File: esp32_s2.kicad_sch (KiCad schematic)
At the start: 15 parts, among them U3 ESP32-S2-MINI-2U-N4

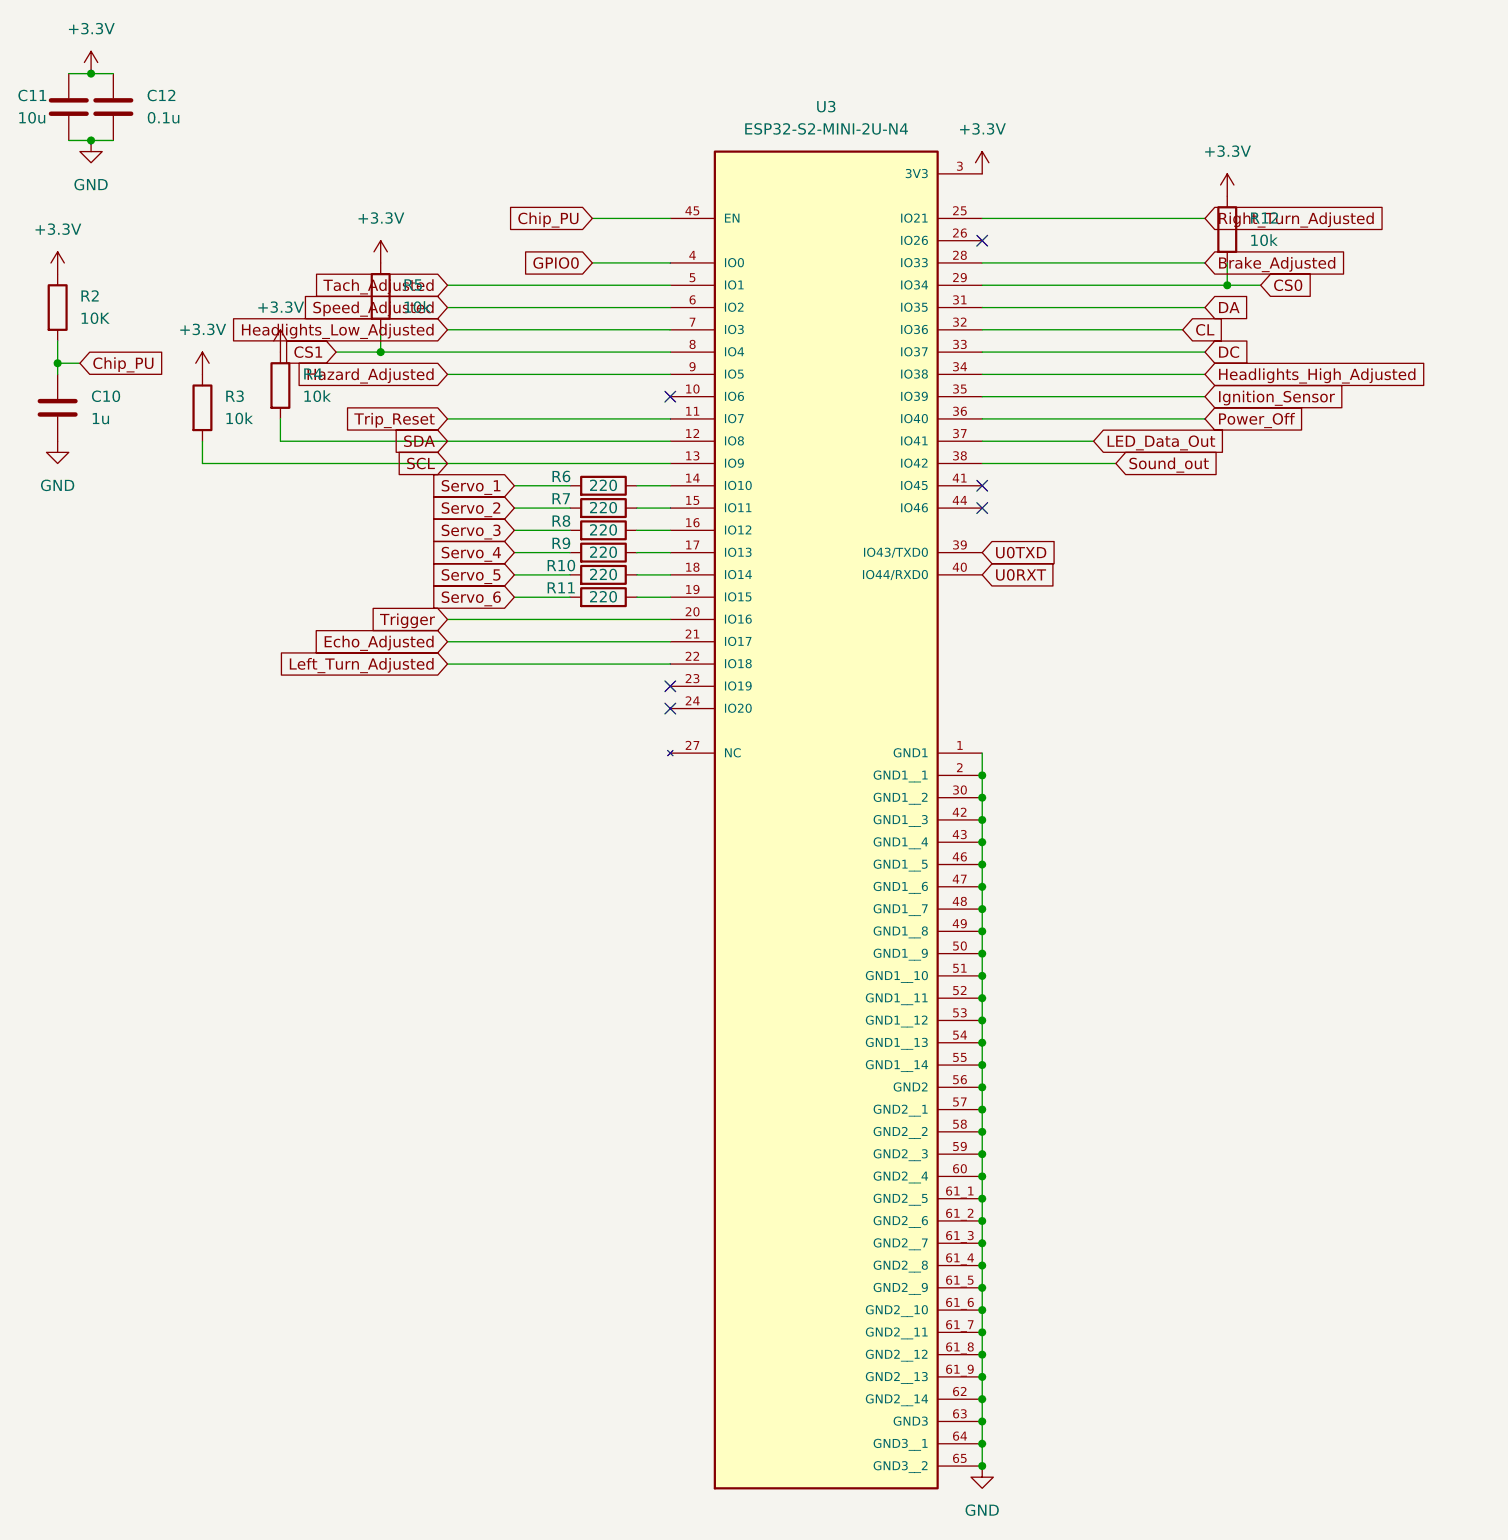
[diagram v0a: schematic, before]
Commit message: Update
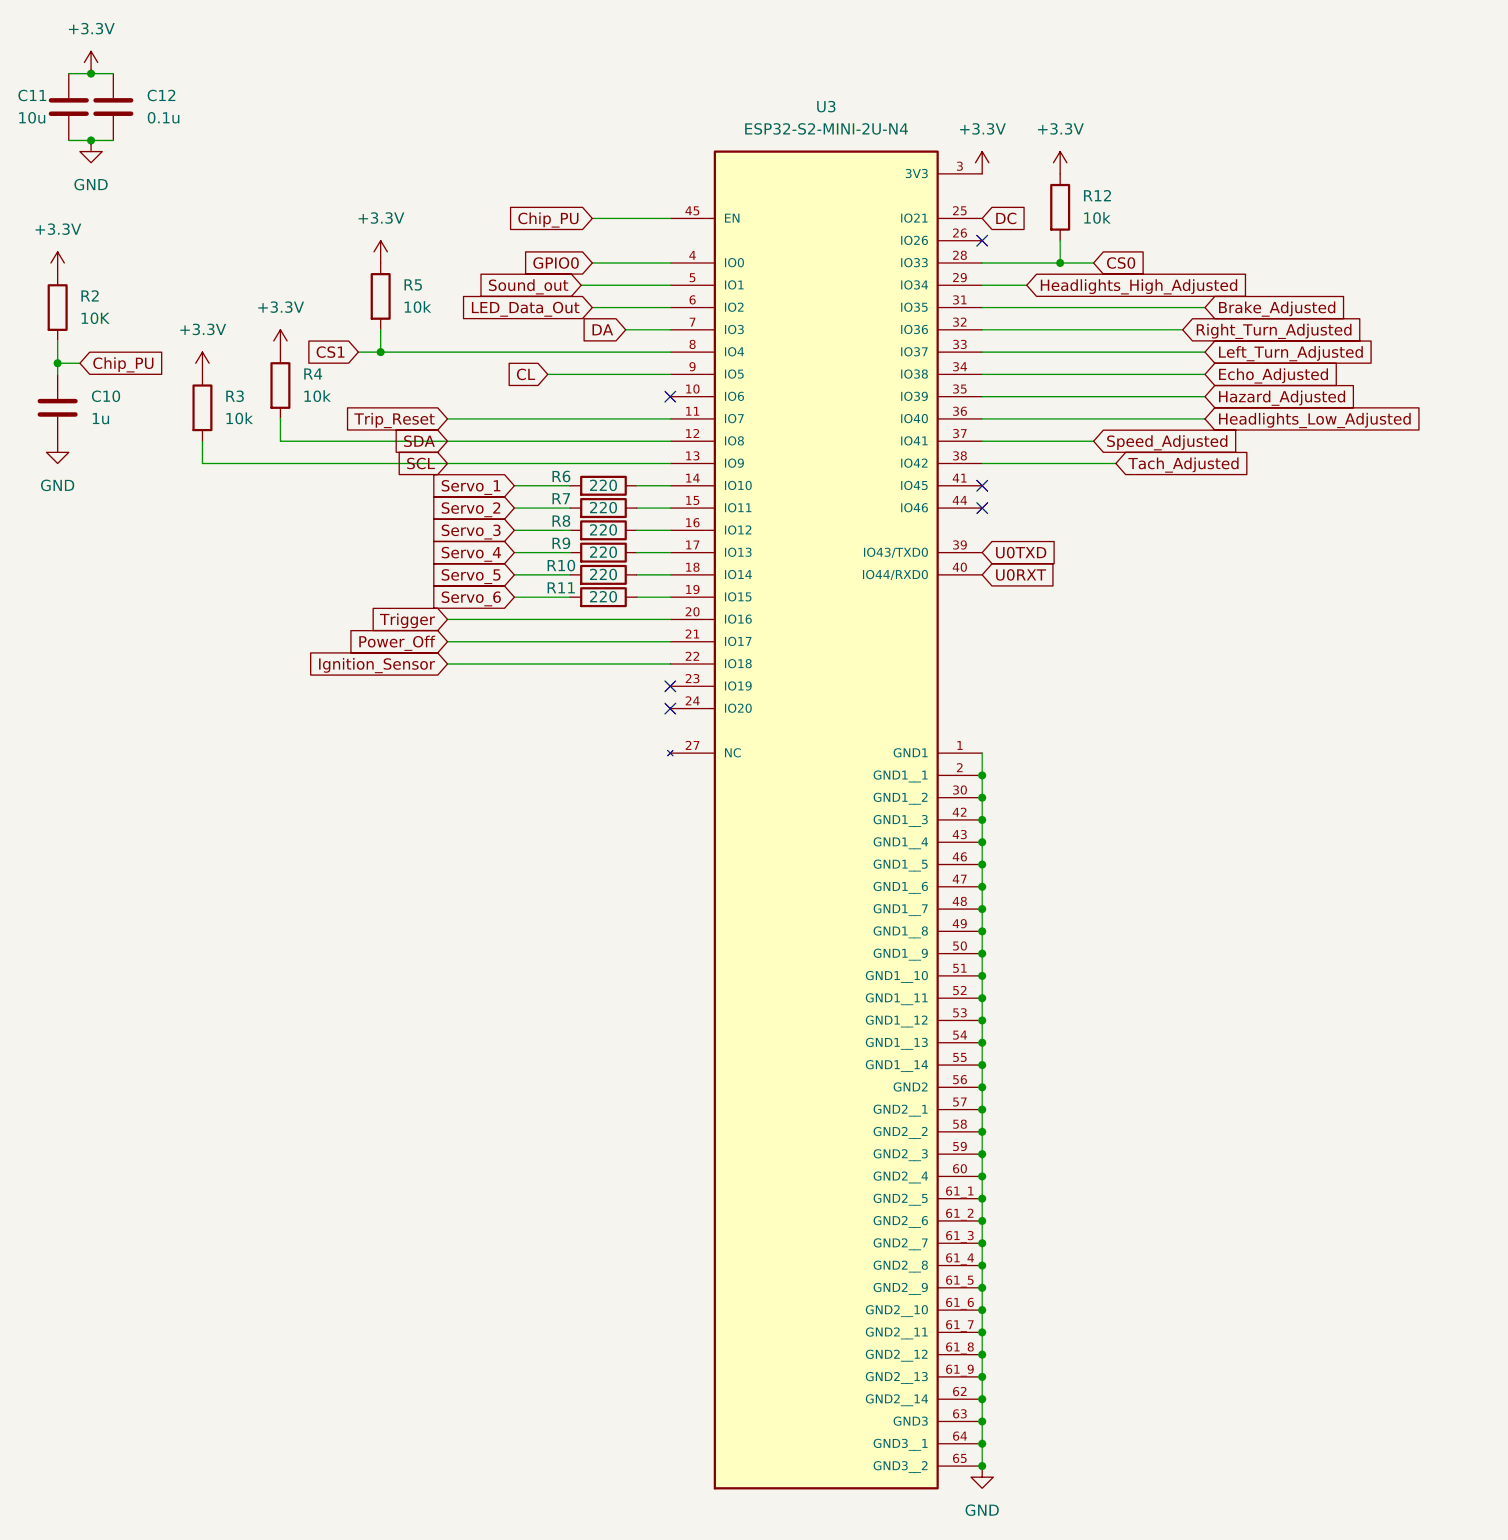
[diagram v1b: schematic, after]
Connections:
- net Brake_Adjusted: now also U3.31 (IO35); no longer U3.28 (IO33)
- net CL: now also U3.9 (IO5); no longer U3.32 (IO36)
- net CS0: now also U3.28 (IO33); no longer U3.29 (IO34)
- net DA: now also U3.7 (IO3); no longer U3.31 (IO35)
- net DC: now also U3.25 (IO21); no longer U3.33 (IO37)
- net Echo_Adjusted: now also U3.34 (IO38); no longer U3.21 (IO17)
- net Hazard_Adjusted: now also U3.35 (IO39); no longer U3.9 (IO5)
- net Headlights_High_Adjusted: now also U3.29 (IO34); no longer U3.34 (IO38)
- net Headlights_Low_Adjusted: now also U3.36 (IO40); no longer U3.7 (IO3)
- net Ignition_Sensor: now also U3.22 (IO18); no longer U3.35 (IO39)
- net LED_Data_Out: now also U3.6 (IO2); no longer U3.37 (IO41)
- net Left_Turn_Adjusted: now also U3.33 (IO37); no longer U3.22 (IO18)
- net Power_Off: now also U3.21 (IO17); no longer U3.36 (IO40)
- net Right_Turn_Adjusted: now also U3.32 (IO36); no longer U3.25 (IO21)
- net Sound_out: now also U3.5 (IO1); no longer U3.38 (IO42)
- net Speed_Adjusted: now also U3.37 (IO41); no longer U3.6 (IO2)
- net Tach_Adjusted: now also U3.38 (IO42); no longer U3.5 (IO1)
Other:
- moved on the sheet: R12

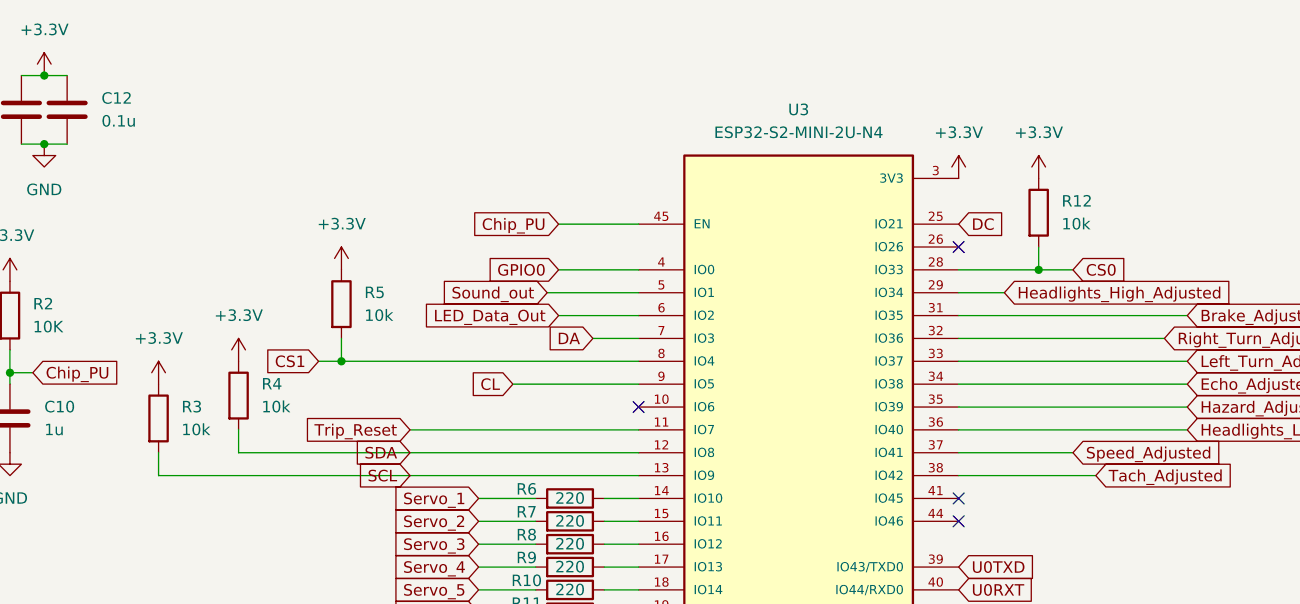
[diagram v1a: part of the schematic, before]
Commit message: update
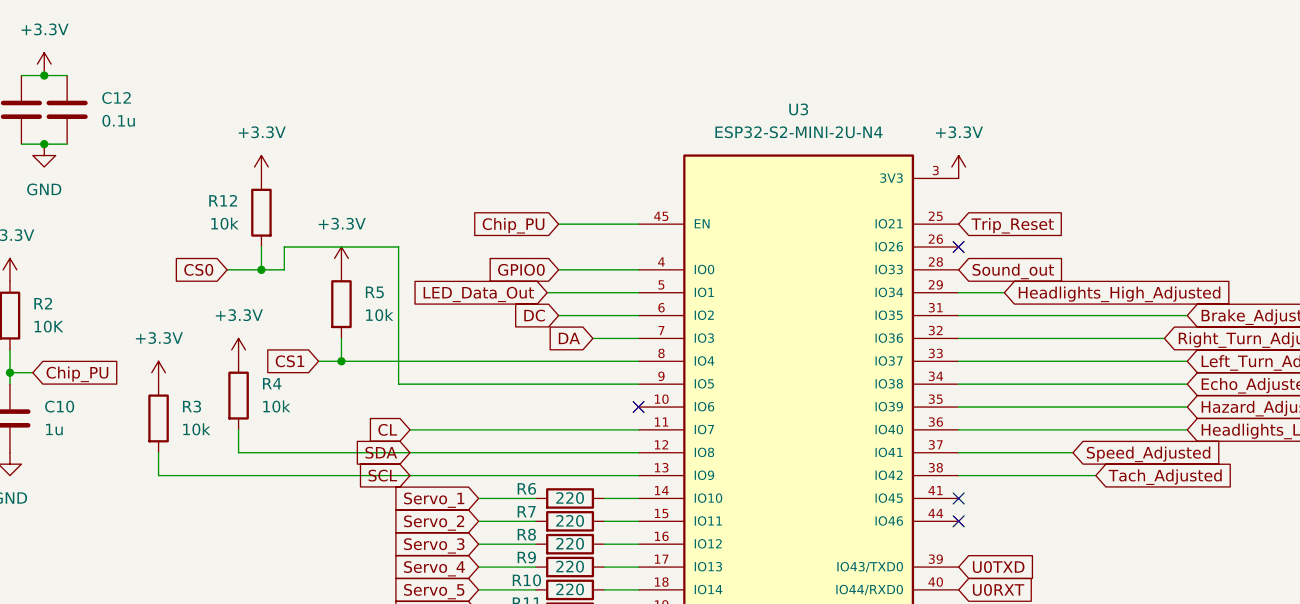
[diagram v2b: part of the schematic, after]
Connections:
- net CL: now also U3.11 (IO7); no longer U3.9 (IO5)
- net CS0: now also U3.9 (IO5); no longer U3.28 (IO33)
- net DC: now also U3.6 (IO2); no longer U3.25 (IO21)
- net LED_Data_Out: now also U3.5 (IO1); no longer U3.6 (IO2)
- net Sound_out: now also U3.28 (IO33); no longer U3.5 (IO1)
- net Trip_Reset: now also U3.25 (IO21); no longer U3.11 (IO7)
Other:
- moved on the sheet: R12
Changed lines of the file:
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@@
 	)
 	(junction
-		(at 132.08 43.18)
-		(diameter 0)
-		(color 0 0 0 0)
-	)
-	(junction
 		(at 123.19 160.02)
 		(diameter 0)
@@
 	)
 	(junction
+		(at 45.72 43.18)
+		(diameter 0)
+		(color 0 0 0 0)
+	)
+	(junction
 		(at 123.19 134.62)
 		(diameter 0)
@@
 	(wire
 		(pts
+			(xy 45.72 43.18) (xy 48.26 43.18)
+		)
+		(stroke
+			(width 0)
+			(type default)
+		)
+	)
+	(wire
+		(pts
 			(xy 123.19 147.32) (xy 123.19 149.86)
 		)
@@
 	(wire
 		(pts
-			(xy 73.66 55.88) (xy 87.63 55.88)
+			(xy 48.26 40.64) (xy 48.26 43.18)
 		)
 		(stroke
@@
 	(wire
 		(pts
-			(xy 132.08 43.18) (xy 123.19 43.18)
+			(xy 60.96 55.88) (xy 60.96 40.64)
 		)
 		(stroke
@@
 	(wire
 		(pts
+			(xy 60.96 40.64) (xy 48.26 40.64)
+		)
+		(stroke
+			(width 0)
+			(type default)
+		)
+	)
+	(wire
+		(pts
 			(xy 128.27 45.72) (xy 123.19 45.72)
 		)
@@
 	(wire
 		(pts
-			(xy 132.08 43.18) (xy 135.89 43.18)
+			(xy 41.91 43.18) (xy 45.72 43.18)
 		)
 		(stroke
@@
 	(wire
 		(pts
-			(xy 132.08 40.64) (xy 132.08 43.18)
+			(xy 60.96 55.88) (xy 87.63 55.88)
 		)
 		(stroke
@@
 		)
 	)
+	(wire
+		(pts
+			(xy 45.72 40.64) (xy 45.72 43.18)
+		)
+		(stroke
+			(width 0)
+			(type default)
+		)
+	)
 	(global_label "Right_Turn_Adjusted"
 		(shape input)
@@
 	(global_label "Trip_Reset"
 		(shape input)
-		(at 62.23 60.96 180)
+		(at 123.19 38.1 0)
 		(fields_autoplaced yes)
 		(effects
@@
 				(size 1.27 1.27)
 			)
-			(justify right)
+			(justify left)
 		)
 		(property "Intersheetrefs" "${INTERSHEET_REFS}"
-			(at 49.5686 60.96 0)
+			(at 135.8514 38.1 0)
 			(hide yes)
 			(show_name no)
@@
 					(size 1.27 1.27)
 				)
-				(justify right)
+				(justify left)
 			)
 		)
@@
 	(global_label "Sound_out"
 		(shape input)
-		(at 77.47 45.72 180)
+		(at 123.19 43.18 0)
 		(fields_autoplaced yes)
 		(effects
@@
 				(size 1.27 1.27)
 			)
-			(justify right)
+			(justify left)
 		)
 		(property "Intersheetrefs" "${INTERSHEET_REFS}"
-			(at 64.688 45.72 0)
+			(at 135.972 43.18 0)
 			(hide yes)
 			(show_name no)
@@
 					(size 1.27 1.27)
 				)
-				(justify right)
+				(justify left)
 			)
 		)
@@
 	(global_label "LED_Data_Out"
 		(shape input)
-		(at 78.74 48.26 180)
+		(at 77.47 45.72 180)
 		(fields_autoplaced yes)
 		(effects
@@
 		)
 		(property "Intersheetrefs" "${INTERSHEET_REFS}"
-			(at 62.8736 48.26 0)
+			(at 61.6036 45.72 0)
 			(hide yes)
 			(show_name no)
@@
 	(global_label "CL"
 		(shape input)
-		(at 73.66 55.88 180)
+		(at 62.23 60.96 180)
 		(fields_autoplaced yes)
 		(effects
@@
 		)
 		(property "Intersheetrefs" "${INTERSHEET_REFS}"
-			(at 68.3767 55.88 0)
+			(at 56.9467 60.96 0)
 			(hide yes)
 			(show_name no)
@@
 	(global_label "DC"
 		(shape input)
-		(at 123.19 38.1 0)
+		(at 78.74 48.26 180)
 		(fields_autoplaced yes)
 		(effects
@@
 				(size 1.27 1.27)
 			)
-			(justify left)
+			(justify right)
 		)
 		(property "Intersheetrefs" "${INTERSHEET_REFS}"
-			(at 128.7152 38.1 0)
+			(at 73.2148 48.26 0)
 			(hide yes)
 			(show_name no)
@@
 					(size 1.27 1.27)
 				)
-				(justify left)
+				(justify right)
 			)
 		)
@@
 	(global_label "CS0"
 		(shape input)
-		(at 135.89 43.18 0)
+		(at 41.91 43.18 180)
 		(fields_autoplaced yes)
 		(effects
@@
 				(size 1.27 1.27)
 			)
-			(justify left)
+			(justify right)
 		)
 		(property "Intersheetrefs" "${INTERSHEET_REFS}"
-			(at 142.5642 43.18 0)
+			(at 35.2358 43.18 0)
 			(hide yes)
 			(show_name no)
@@
 					(size 1.27 1.27)
 				)
-				(justify left)
+				(justify right)
 			)
 		)
@@
 	(symbol
 		(lib_id "power:+3.3V")
-		(at 132.08 33.02 0)
+		(at 45.72 33.02 0)
+		(mirror y)
 		(unit 1)
 		(body_style 1)
@@
 		(fields_autoplaced yes)
 		(property "Reference" "#PWR057"
-			(at 132.08 36.83 0)
+			(at 45.72 36.83 0)
 			(hide yes)
 			(show_name no)
@@
 		)
 		(property "Value" "+3.3V"
-			(at 132.08 27.94 0)
+			(at 45.72 27.94 0)
 			(show_name no)
 			(do_not_autoplace no)
@@
 		)
 		(property "Footprint" ""
-			(at 132.08 33.02 0)
+			(at 45.72 33.02 0)
 			(hide yes)
 			(show_name no)
@@
 		)
 		(property "Datasheet" ""
-			(at 132.08 33.02 0)
+			(at 45.72 33.02 0)
 			(hide yes)
 			(show_name no)
@@
 		)
 		(property "Description" "Power symbol creates a global label with name \"+3.3V\""
-			(at 132.08 33.02 0)
+			(at 45.72 33.02 0)
 			(hide yes)
 			(show_name no)
@@
 	(symbol
 		(lib_id "Device:R")
-		(at 132.08 36.83 0)
+		(at 45.72 36.83 0)
+		(mirror y)
 		(unit 1)
 		(body_style 1)
@@
 		(fields_autoplaced yes)
 		(property "Reference" "R12"
-			(at 134.62 35.5599 0)
+			(at 43.18 35.5599 0)
 			(show_name no)
 			(do_not_autoplace no)
@@
 		)
 		(property "Value" "10k"
-			(at 134.62 38.0999 0)
+			(at 43.18 38.0999 0)
 			(show_name no)
 			(do_not_autoplace no)
@@
 		)
 		(property "Footprint" "Resistor_THT:R_Axial_DIN0207_L6.3mm_D2.5mm_P10.16mm_Horizontal"
-			(at 130.302 36.83 90)
+			(at 47.498 36.83 90)
 			(hide yes)
 			(show_name no)
@@
 		)
 		(property "Datasheet" ""
-			(at 132.08 36.83 0)
+			(at 45.72 36.83 0)
 			(hide yes)
 			(show_name no)
@@
 		)
 		(property "Description" "Resistor"
-			(at 132.08 36.83 0)
+			(at 45.72 36.83 0)
 			(hide yes)
 			(show_name no)
